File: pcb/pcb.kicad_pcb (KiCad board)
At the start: 2 copper layers, 33 x 40.6 mm, 12 parts, among them J1 Conn_01x15 Right, J2 Conn_01x15 Left, J3 DIN41612_02x08_AB_EvenPins, P1 Conn_01x06, U1 STM32F756VGTx, U2 MP34DT05-A, U3 ISM330DHCX

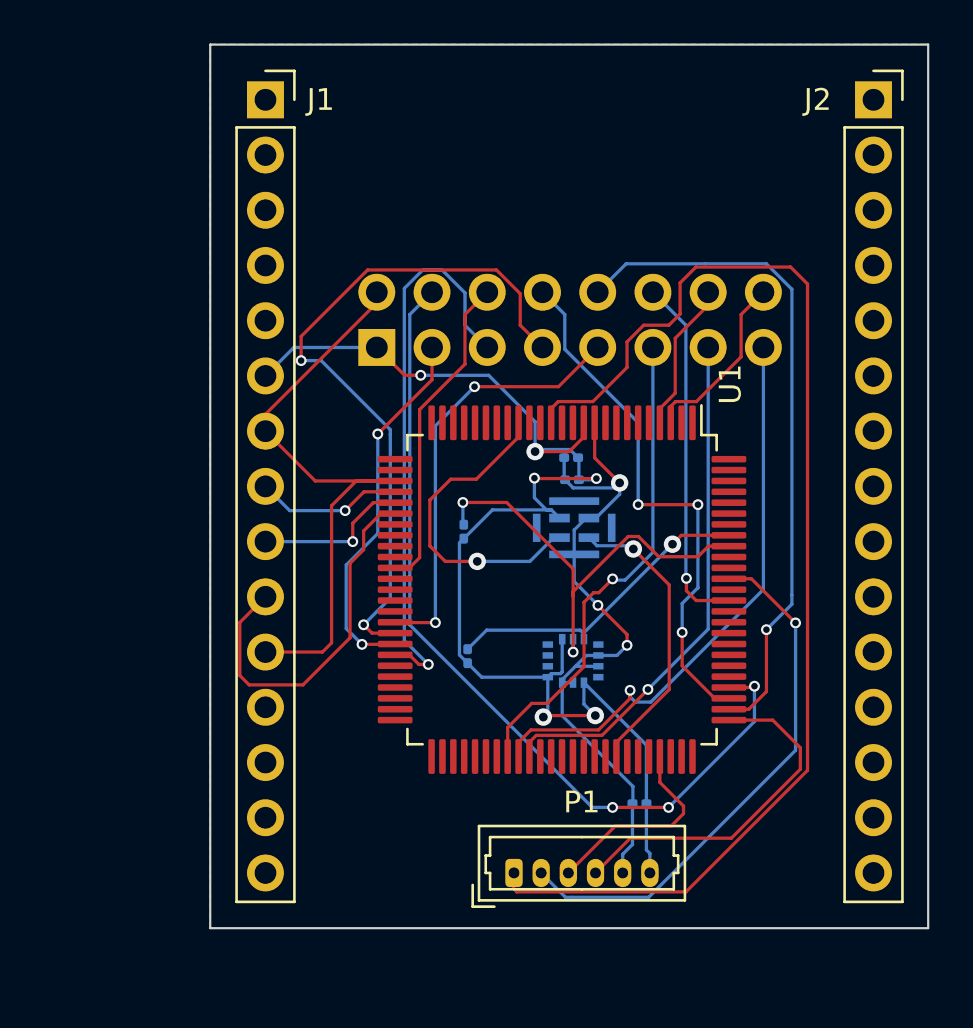
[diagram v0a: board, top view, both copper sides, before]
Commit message: pcb_8
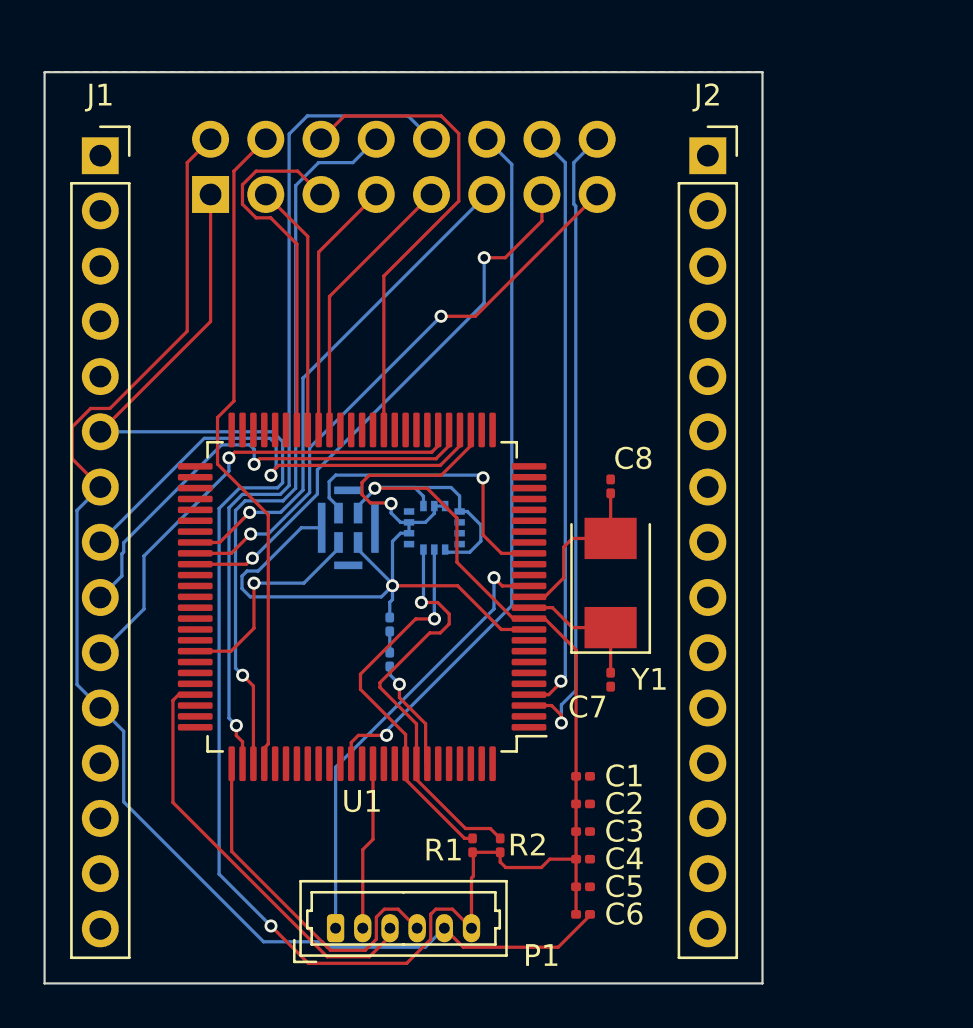
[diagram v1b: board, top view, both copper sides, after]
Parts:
- added C4: 100nF, Capacitor_SMD:C_0201_0603Metric, F.Cu at (113.7, 128.9)
- added C5: 100nF, Capacitor_SMD:C_0201_0603Metric, F.Cu at (113.7, 130.2)
- added C6: 100nF, Capacitor_SMD:C_0201_0603Metric, F.Cu at (113.7, 131.4)
- added C7: 1pF, Capacitor_SMD:C_0201_0603Metric, F.Cu at (114.9, 120.7)
- added C8: 1pF, Capacitor_SMD:C_0201_0603Metric, F.Cu at (114.9, 111.8)
- added D1: LED, Diode_SMD:D_0201_0603Metric, B.Cu at (104.8, 118.1)
- added R3: 680ohm, Resistor_SMD:R_0201_0603Metric, B.Cu at (104.8, 119.7)
- added Y1: Crystal, Crystal:Crystal_SMD_Abracon_ABM3-2Pin_5.0x3.2mm, F.Cu at (114.9, 116.2)
- C1, C2, C3, R1, R2: moved to F.Cu
- moved C3 16.2 mm to (113.7, 127.6), turned to 0 degrees
- moved C2 15.9 mm to (113.7, 126.4), turned to 0 degrees
- moved R1 14.4 mm to (108.6, 128.3)
- moved J3 10.4 mm to (96.5, 98.3)
- moved U2 10.4 mm to (102.9, 113.7), turned to 0 degrees
- moved U1 9.20 mm to (103.5, 116.8), turned to 180 degrees
- moved U3 8.84 mm to (106.8, 113.7), turned to 0 degrees
- moved R2 8.83 mm to (109.9, 128.3)
- moved P1 8.59 mm to (102.3, 132.1)
- moved J2 8.04 mm to (119.4, 96.5)
- moved J1 8.02 mm to (91.5, 96.5)
- moved C1 2.88 mm to (113.7, 125.1), turned to 0 degrees
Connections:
- U1 pad 12: unconnected-(U1-Pad12) -> /OSC_IN
- U1 pad 13: unconnected-(U1-Pad13) -> /OSC_OUT
- U1 pad 94: unconnected-(U1-Pad94) -> /boot0
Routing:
- net VDD: track 61.1 -> 106.7 mm, vias 6 -> 2
- net GND: track 60.6 -> 100.4 mm, vias 3 -> 2
- net /NRST: track 56.0 -> 20.9 mm, vias 0 -> 1
- net /SAI1_FS: track 8.33 -> 29.6 mm, vias 0 -> 1
- net /SPI4_SCK: track 32.3 -> 11.9 mm, vias 2 -> 0
- net /SAI1_SCK: track 6.92 -> 27.2 mm, vias 0 -> 1
- net /SWO: track 24.7 -> 7.76 mm, vias 1 -> 0
- net /SAI1_SD: track 16.5 -> 33.0 mm
- net /SPI1_SCK: track 6.79 -> 21.7 mm
- net /SPI1_MISO: track 7.20 -> 21.6 mm
- net /SWDIO: track 9.51 -> 19.5 mm
- net /SPI4_MOSI: track 26.0 -> 17.0 mm, vias 1 -> 0
- net /SPI3_MISO: track 39.6 -> 30.7 mm, vias 3 -> 0
- net /SPI3_SCK: track 24.8 -> 33.7 mm, vias 3 -> 1
- net /OSC_OUT: track 0.00 -> 7.77 mm
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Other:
- board size 33 x 40.6 mm -> 33 x 41.9 mm
